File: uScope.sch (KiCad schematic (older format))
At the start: 32 parts, among them J1 Pump+, J2 Pump-, J3 U_E, J4 U_F, J5 Conn_01x02, J6 U_K, J7 Anode, U1 K, U2 E, U3 F, U4 Pump, U6 RHV2-1212S/R20

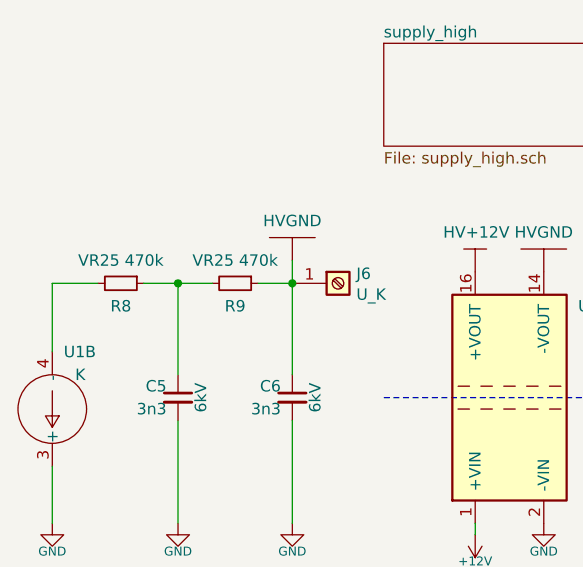
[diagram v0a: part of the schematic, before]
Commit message: - PCB WiP
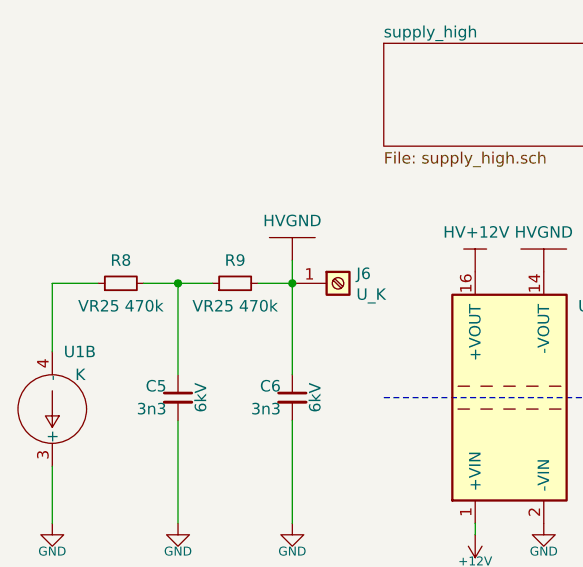
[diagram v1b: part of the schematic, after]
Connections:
- net HVGND: now also R9.2; no longer R9.1
- net at U1.4 (-): now also R8.1; no longer R8.2
- new net: C5.1, R8.2, R9.1
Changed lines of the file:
@@
 F 6 "0.6" V 1050 3750 50  0001 C CNN "Price [PLN]"
 	1    1050 3750
-	0    1    1    0
+	0    -1   -1   0
 $EndComp
 $Comp
@@
 F 6 "0.6" V 1550 3750 50  0001 C CNN "Price [PLN]"
 	1    1550 3750
-	0    1    1    0
+	0    -1   -1   0
 $EndComp
 $Sheet
